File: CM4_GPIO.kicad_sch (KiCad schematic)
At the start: 34 parts, among them IC5 74LVC1G07QSE-7, J3 2222, SW1 SW_Push, SW2 SW_Push, SW3 SW_Push

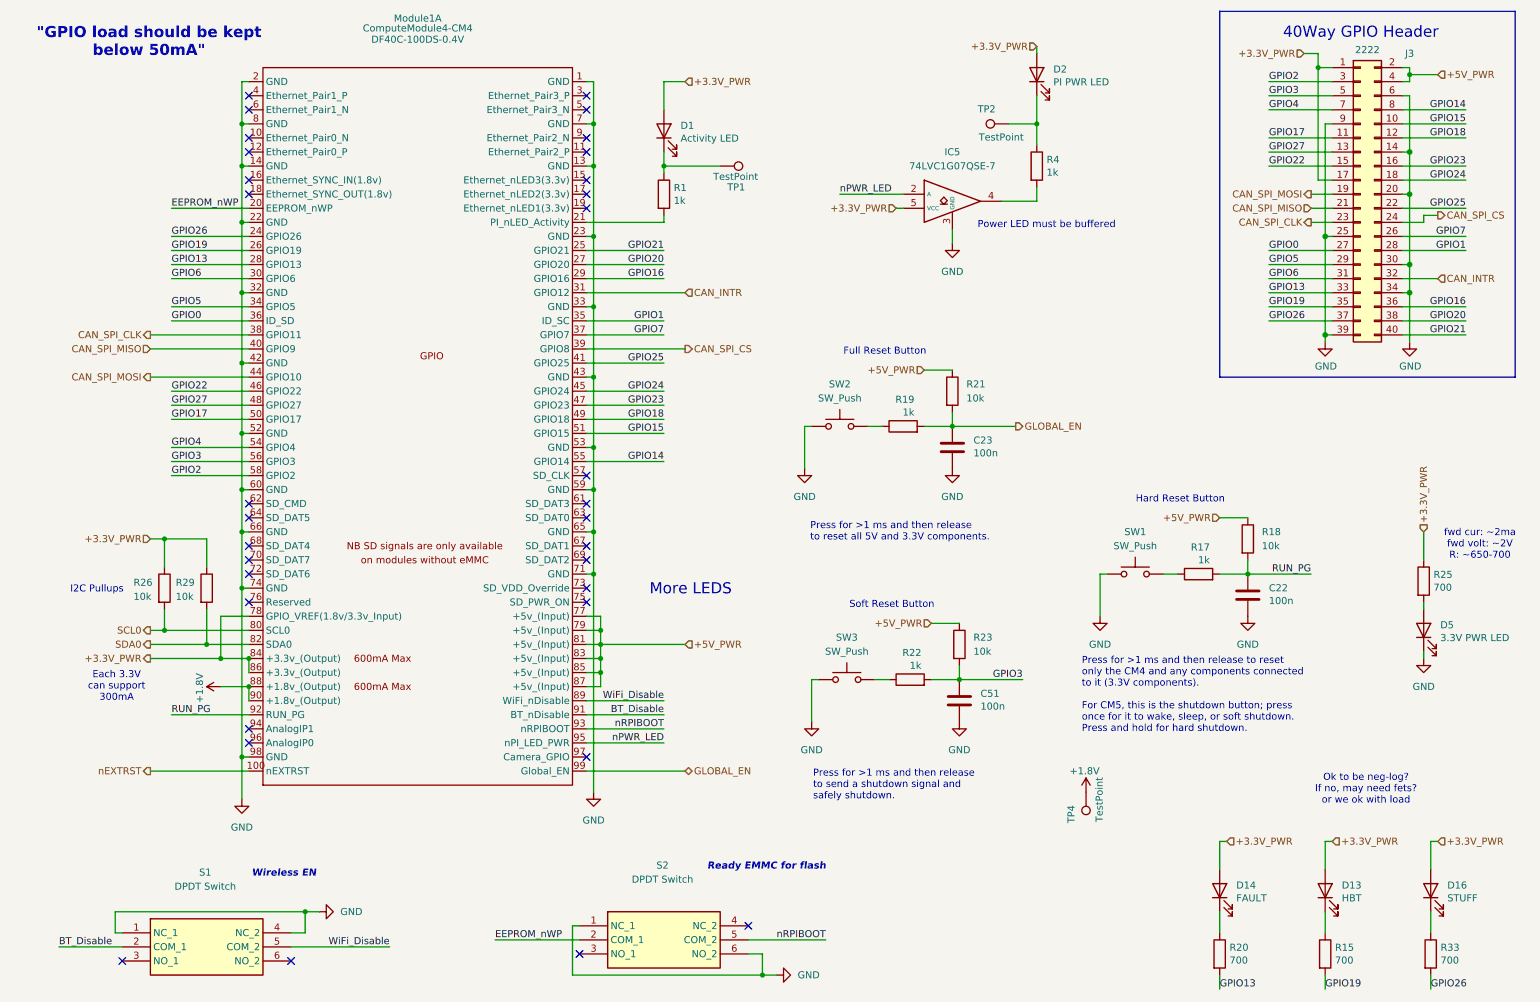
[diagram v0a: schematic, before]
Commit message: my life is horrible
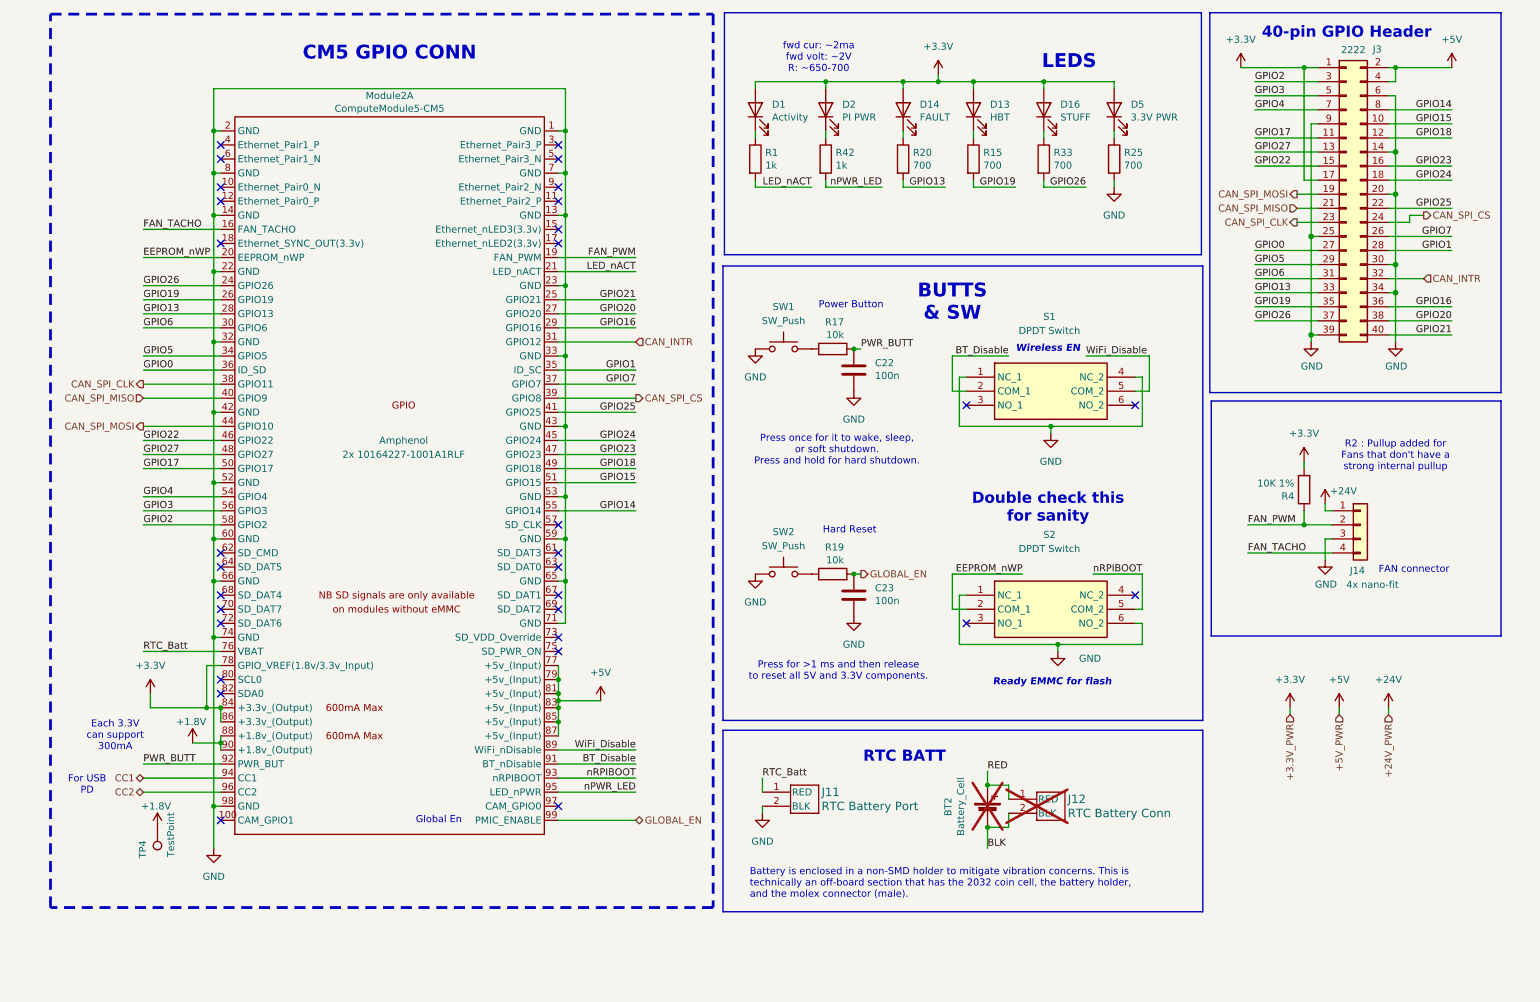
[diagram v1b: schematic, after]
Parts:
- removed C51: 100n, Capacitor_SMD:C_0603_1608Metric, symbol Device:C
- removed IC5: 74LVC1G07QSE-7, Controls_Pi:SOT65P210X110-5N, symbol 74LVC1G07QSE-7:74LVC1G07QSE-7
- removed Module1: ComputeModule4-CM4, CM4IO:Raspberry-Pi-4-Compute-Module, symbol CM4IO:ComputeModule4-CM4
- removed R18, R21, R23, R26, R29: 10k, Resistor_SMD:R_0603_1608Metric, symbol Device:R
- removed R22: 1k, Resistor_SMD:R_0603_1608Metric, symbol Device:R
- removed SW3: SW_Push, Button_Switch_SMD:SW_SPST_B3SL-1002P, symbol Switch:SW_Push
- removed TP1, TP2: TestPoint, TestPoint:TestPoint_Pad_2.0x2.0mm, symbol Connector:TestPoint
- added BT2: Battery_Cell, symbol Device:Battery_Cell
- added J11: RTC Battery Port, Controls_Pi:CONN02_530470210_MOL, symbol 530470210:530470210
- added J12: RTC Battery Conn, Controls_Pi:CONN02_530470210_MOL, symbol 530470210:530470210
- added J14: 4x nano-fit, Connector_JST:JST_SH_BM04B-SRSS-TB_1x04-1MP_P1.00mm_Vertical, symbol Connector_Generic:Conn_01x04
- added Module2: ComputeModule5-CM5, CM5IO:Raspberry-Pi-5-Compute-Module, symbol CM5IO:ComputeModule5-CM5
- added R42: 1k, Resistor_SMD:R_0603_1608Metric, symbol Device:R
- D1: value Activity LED -> Activity
- D2: value PI PWR LED -> PI PWR
- D5: value 3.3V PWR LED -> 3.3V PWR
- R17, R19: value 1k -> 10k
- R4: value 1k -> 10K 1%; Field4 (none) -> Farnell; Field6 (none) -> MCR01MZPF1002; Field7 (none) -> Rohm; P/N CRCW08051K00FKEAC -> (none); Part Description (none) -> Resistor 10K M1005 1% 63mW
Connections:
- net +1.8V: now also Module2.88 (+1.8v_(Output)), Module2.90 (+1.8v_(Output))
- net BT_Disable: now also Module2.91 (BT_nDisable)
- net CAN_INTR: now also Module2.31 (GPIO12)
- net CAN_SPI_CLK: now also Module2.38 (GPIO11)
- net CAN_SPI_CS: now also Module2.39 (GPIO8)
- net CAN_SPI_MISO: now also Module2.40 (GPIO9)
- net CAN_SPI_MOSI: now also Module2.44 (GPIO10)
- net EEPROM_nWP: now also Module2.20 (EEPROM_nWP)
- net GLOBAL_EN: now also Module2.99 (PMIC_ENABLE)
- net GND: now also R25.2, J11.2 (BLK), J14.3 (Pin_3), Module2.1 (GND), Module2.13 (GND), Module2.14 (GND), Module2.2 (GND), Module2.22 (GND), Module2.23 (GND), Module2.32 (GND), Module2.33 (GND), Module2.42 (GND), Module2.43 (GND), Module2.52 (GND), Module2.53 (GND), Module2.59 (GND), Module2.60 (GND), Module2.65 (GND), Module2.66 (GND), Module2.7 (GND), Module2.71 (GND), Module2.74 (GND), Module2.8 (GND), Module2.98 (GND); no longer D5.1 (K)
- net GPIO0: now also Module2.36 (ID_SD)
- net GPIO1: now also Module2.35 (ID_SC)
- net GPIO13: now also Module2.28 (GPIO13)
- net GPIO14: now also Module2.55 (GPIO14)
- net GPIO15: now also Module2.51 (GPIO15)
- net GPIO16: now also Module2.29 (GPIO16)
- net GPIO17: now also Module2.50 (GPIO17)
- net GPIO18: now also Module2.49 (GPIO18)
- net GPIO19: now also Module2.26 (GPIO19)
- net GPIO2: now also Module2.58 (GPIO2)
- net GPIO20: now also Module2.27 (GPIO20)
- net GPIO21: now also Module2.25 (GPIO21)
- net GPIO22: now also Module2.46 (GPIO22)
- net GPIO23: now also Module2.47 (GPIO23)
- net GPIO24: now also Module2.45 (GPIO24)
- net GPIO25: now also Module2.41 (GPIO25)
- net GPIO26: now also Module2.24 (GPIO26)
- net GPIO27: now also Module2.48 (GPIO27)
- net GPIO3: now also Module2.56 (GPIO3)
- net GPIO4: now also Module2.54 (GPIO4)
- net GPIO5: now also Module2.34 (GPIO5)
- net GPIO6: now also Module2.30 (GPIO6)
- net GPIO7: now also Module2.37 (GPIO7)
- net WiFi_Disable: now also Module2.89 (WiFi_nDisable)
- net nPWR_LED: now also Module2.95 (LED_nPWR), R42.2
- net nRPIBOOT: now also Module2.93 (nRPIBOOT)
- net +3.3V: now reaches D5.2 (A)
- net +3.3V: now also D1.2 (A), D13.2 (A), D14.2 (A), D16.2 (A), D2.2 (A), J3.1 (Pin_1), J3.17 (Pin_17), R4.2, Module2.78 (GPIO_VREF(1.8v/3.3v_Input)), Module2.84 (+3.3v_(Output)), Module2.86 (+3.3v_(Output)); no longer R25.2
- net at D2.1 (K): now also R42.1; no longer R4.1
- net LED_nACT: now reaches R1.2
- net LED_nACT: now also Module2.21 (LED_nACT)
- removed net +3.3V_PWR: D1.2 (A), D13.2 (A), D14.2 (A), D16.2 (A), D2.2 (A), J3.1 (Pin_1), J3.17 (Pin_17), R25.1
- net +5V_PWR renamed +5V
- net +5V: now also Module2.77 (+5v_(Input)), Module2.79 (+5v_(Input)), Module2.81 (+5v_(Input)), Module2.83 (+5v_(Input)), Module2.85 (+5v_(Input)), Module2.87 (+5v_(Input))
- net RUN_PG renamed PWR_BUTT
- net PWR_BUTT: now also Module2.92 (PWR_BUT)
- new net: D5.1 (K), R25.1
- new net +24V: J14.1 (Pin_1)
- new net BLK: BT2.2 (-), J12.2 (BLK)
- new net CC1: Module2.94 (CC1)
- new net CC2: Module2.96 (CC2)
- new net FAN_PWM: J14.2 (Pin_2), Module2.19 (FAN_PWM), R4.1
- new net FAN_TACHO: J14.4 (Pin_4), Module2.16 (FAN_TACHO)
- new net RED: BT2.1 (+), J12.1 (RED)
- new net RTC_Batt: J11.1 (RED), Module2.76 (VBAT)
- no-connect marks 33 -> 31
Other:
- note added: "40-pin GPIO Header"
- note added: "BUTTS & SW"
- note added: "Battery is enclosed in a non-SMD holder to mitigate vibration concerns. This is technically an off-board section that has the 2032 coin cell, the battery holder, and the molex connector (male)."
- note added: "CM5 GPIO CONN"
- note added: "Double check this for sanity"
- note added: "FAN connector"
- note added: "For USB PD"
- note added: "Global En"
- note added: "Hard Reset"
- note added: "LEDS"
- note added: "Power Button"
- note added: "Press once for it to wake, sleep, or soft shutdown. Press and hold for hard shutdown."
- note added: "R2 : Pullup added for Fans that don't have a strong internal pullup"
- note added: "RTC BATT"
- note removed: ""GPIO load should be kept below 50mA""
- note removed: "40Way GPIO Header"
- note removed: "Full Reset Button"
- note removed: "Hard Reset Button"
- note removed: "I2C Pullups"
- note removed: "More LEDS"
- note removed: "Ok to be neg-log? If no, may need fets? or we ok with load"
- note removed: "Power LED must be buffered"
- note removed: "Press for >1 ms and then release to reset only the CM4 and any components connected to it (3.3V components). For CM5, this is the shutdown button; press once for it to wake, sleep, or soft shutdown. Press and hold for hard shutdown."
- note removed: "Press for >1 ms and then release to send a shutdown signal and safely shutdown."
- note removed: "Soft Reset Button"
- moved on the sheet: C22, C23, D13, D14, D16, D5, J3, R15, R17, R19, R20, R25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
